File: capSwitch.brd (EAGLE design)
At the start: 45.4 x 45.7 mm, 10 parts, among them T1 2N2222, T2 2N2222

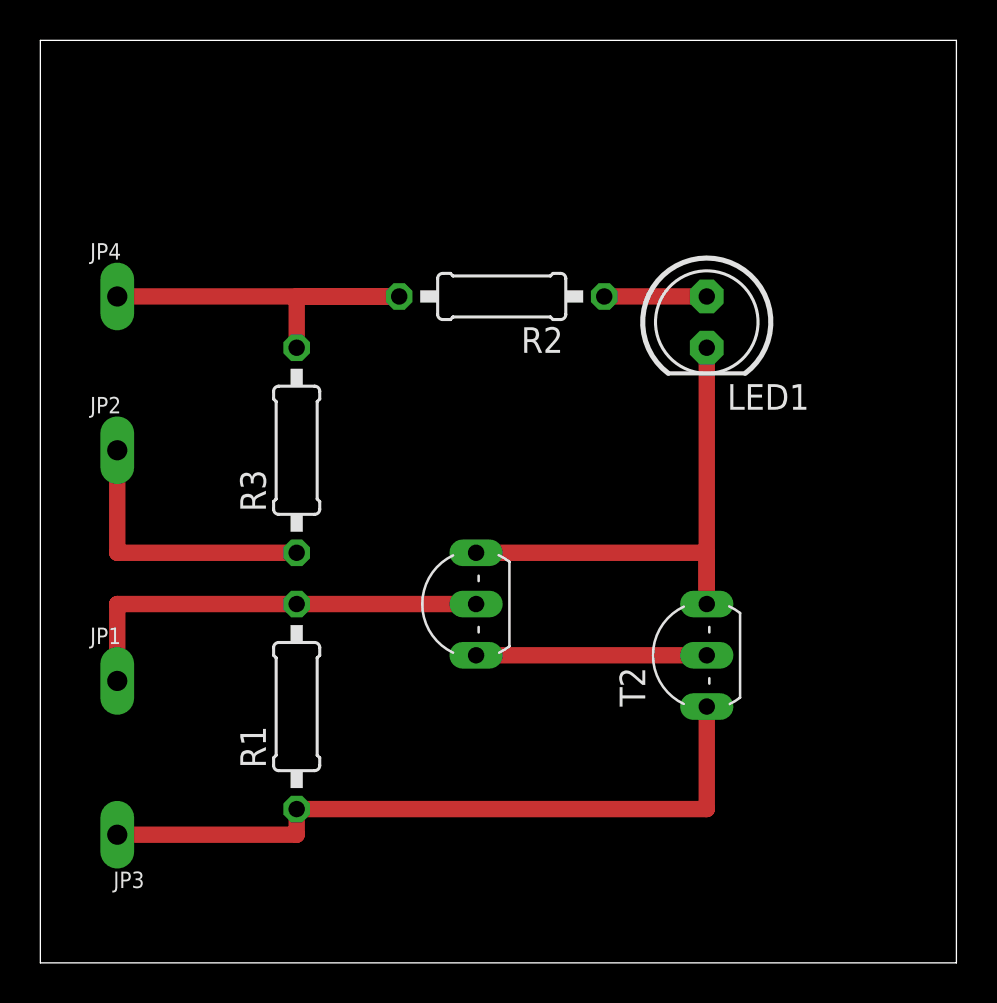
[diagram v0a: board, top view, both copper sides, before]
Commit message: refined board, ready to be etched
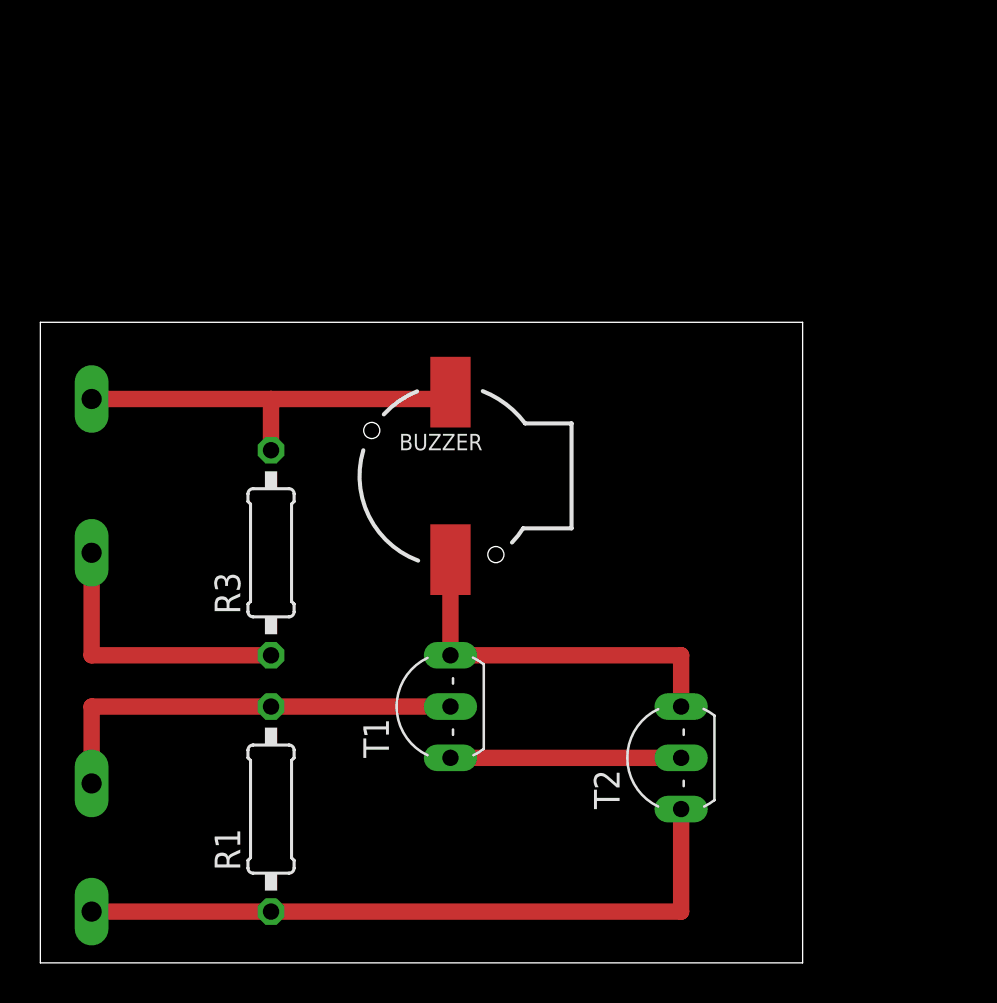
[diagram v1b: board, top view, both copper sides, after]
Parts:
- removed LED1: (no value), adafruit:LED5MM
- removed R2: 220, dp_devices:RTH025W
- added BUZZER: BUZZERSMD2-KIT, SparkFun-Electromechanical:BUZZER-CCV-KIT
- moved JP4 5.24 mm to (2.54, 27.9)
- moved T1 5.24 mm to (19.1, 12.7)
- moved JP1 5.24 mm to (2.54, 8.89)
- moved T2 5.24 mm to (30.5, 10.2)
- moved R1 5.24 mm to (11.4, 7.62)
- moved JP2 5.24 mm to (2.54, 20.3)
- moved R3 5.24 mm to (11.4, 20.3)
- moved JP3 4.02 mm to (2.54, 2.54)
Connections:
- removed net N$1: LED1.A, R2.1
- net N$2: now also BUZZER.-; no longer LED1.K
- net VCC: now also BUZZER.+; no longer R2.2
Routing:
- net N$2: track 26.7 -> 18.7 mm
- net N$1: track 5.08 -> 0.00 mm
- net GND: track 35.6 -> 34.3 mm
- net VCC: track 21.6 -> 20.7 mm
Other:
- board size 45.4 x 45.7 mm -> 37.8 x 31.7 mm
- board text added: "BUZZER"
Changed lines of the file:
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@@
 <board>
 <plain>
-<wire x1="0" y1="0" x2="45.39" y2="0" width="0" layer="20"/>
-<wire x1="45.39" y1="0" x2="45.39" y2="45.71" width="0" layer="20"/>
-<wire x1="45.39" y1="45.71" x2="0" y2="45.71" width="0" layer="20"/>
-<wire x1="0" y1="45.71" x2="0" y2="0" width="0" layer="20"/>
+<wire x1="0" y1="0" x2="37.77" y2="0" width="0" layer="20"/>
+<wire x1="37.77" y1="0" x2="37.77" y2="31.74" width="0" layer="20"/>
+<wire x1="37.77" y1="31.74" x2="0" y2="31.74" width="0" layer="20"/>
+<wire x1="0" y1="31.74" x2="0" y2="0" width="0" layer="20"/>
+<text x="17.78" y="25.4" size="0.8128" layer="21">BUZZER</text>
 </plain>
 <attributes>
@@
 </autorouter>
 <elements>
-<element name="JP1" library="microbuilder" package="1X01_OVAL" value="probe_a" x="3.81" y="13.97"/>
-<element name="JP2" library="microbuilder" package="1X01_OVAL" value="probe_b" x="3.81" y="25.4"/>
-<element name="JP3" library="microbuilder" package="1X01_OVAL" value="gnd" x="3.81" y="6.35" rot="R180"/>
-<element name="JP4" library="microbuilder" package="1X01_OVAL" value="vcc" x="3.81" y="33.02"/>
-<element name="LED1" library="adafruit" package="LED5MM" value="" x="33.02" y="31.75" smashed="yes" rot="R270">
-<attribute name="NAME" x="38.1" y="28.6766" size="1.27" layer="25" ratio="10" rot="R180"/>
-<attribute name="VALUE" x="31.2166" y="28.5496" size="1.27" layer="27" ratio="10" rot="R270"/>
-</element>
-<element name="R1" library="dp_devices" package="RTH025W" value="10M" x="12.7" y="12.7" rot="R90"/>
-<element name="R2" library="dp_devices" package="RTH025W" value="220" x="22.86" y="33.02" smashed="yes" rot="R180">
-<attribute name="NAME" x="25.908" y="31.496" size="1.27" layer="25" font="vector" ratio="10" rot="R180"/>
-<attribute name="VALUE" x="22.225" y="35.8775" size="1.27" layer="27" font="vector" ratio="10" rot="R180"/>
-</element>
-<element name="R3" library="dp_devices" package="RTH025W" value="1k" x="12.7" y="25.4" rot="R90"/>
-<element name="T1" library="adafruit" package="TO92-EBC-OVAL" value="2N2222" x="20.32" y="17.78" smashed="yes" rot="R90">
-<attribute name="VALUE" x="25.4" y="14.097" size="1.27" layer="27" ratio="10" rot="R180"/>
-</element>
-<element name="T2" library="adafruit" package="TO92-EBC-OVAL" value="2N2222" x="31.75" y="15.24" rot="R90"/>
+<element name="JP1" library="microbuilder" package="1X01_OVAL" value="probe_a" x="2.54" y="8.89" smashed="yes">
+<attribute name="VALUE" x="1.27" y="10.795" size="0.8128" layer="27" ratio="10"/>
+</element>
+<element name="JP2" library="microbuilder" package="1X01_OVAL" value="probe_b" x="2.54" y="20.32" smashed="yes">
+<attribute name="VALUE" x="5.715" y="18.415" size="0.8128" layer="27" ratio="10" rot="R180"/>
+</element>
+<element name="JP3" library="microbuilder" package="1X01_OVAL" value="gnd" x="2.54" y="2.54" smashed="yes" rot="R180">
+<attribute name="VALUE" x="3.81" y="5.08" size="0.8128" layer="27" ratio="10" rot="R180"/>
+</element>
+<element name="JP4" library="microbuilder" package="1X01_OVAL" value="vcc" x="2.54" y="27.94" smashed="yes">
+<attribute name="VALUE" x="3.81" y="26.67" size="0.8128" layer="27" ratio="10"/>
+</element>
+<element name="R1" library="dp_devices" package="RTH025W" value="10M" x="11.43" y="7.62" rot="R90"/>
+<element name="R3" library="dp_devices" package="RTH025W" value="1k" x="11.43" y="20.32" rot="R90"/>
+<element name="T1" library="adafruit" package="TO92-EBC-OVAL" value="2N2222" x="19.05" y="12.7" rot="R90"/>
+<element name="T2" library="adafruit" package="TO92-EBC-OVAL" value="2N2222" x="30.48" y="10.16" rot="R90"/>
+<element name="BUZZER" library="SparkFun-Electromechanical" package="BUZZER-CCV-KIT" value="BUZZERSMD2-KIT" x="20.32" y="24.13" rot="R90"/>
 </elements>
 <signals>
 <signal name="VCC">
 <contactref element="R3" pad="2"/>
-<contactref element="R2" pad="2"/>
 <contactref element="JP4" pad="1"/>
-<wire x1="3.81" y1="33.02" x2="17.78" y2="33.02" width="0.8128" layer="1"/>
-<wire x1="17.78" y1="33.02" x2="12.7" y2="33.02" width="0.8128" layer="1"/>
-<wire x1="12.7" y1="33.02" x2="12.7" y2="30.48" width="0.8128" layer="1"/>
-</signal>
-<signal name="N$1">
-<contactref element="LED1" pad="A"/>
-<contactref element="R2" pad="1"/>
-<wire x1="33.02" y1="33.02" x2="27.94" y2="33.02" width="0.8128" layer="1"/>
+<contactref element="BUZZER" pad="+"/>
+<wire x1="2.54" y1="27.94" x2="11.43" y2="27.94" width="0.8128" layer="1"/>
+<wire x1="11.43" y1="27.94" x2="11.43" y2="25.4" width="0.8128" layer="1"/>
+<wire x1="11.43" y1="27.94" x2="20.32" y2="27.94" width="0.8128" layer="1"/>
+<wire x1="20.32" y1="27.94" x2="20.32" y2="28.28" width="0.8128" layer="1"/>
 </signal>
 <signal name="GND">
@@
 <contactref element="T2" pad="E"/>
 <contactref element="R1" pad="1"/>
-<wire x1="12.7" y1="7.62" x2="33.02" y2="7.62" width="0.8128" layer="1"/>
-<wire x1="33.02" y1="7.62" x2="33.02" y2="12.7" width="0.8128" layer="1"/>
-<wire x1="12.7" y1="7.62" x2="12.7" y2="6.35" width="0.8128" layer="1"/>
-<wire x1="12.7" y1="6.35" x2="3.81" y2="6.35" width="0.8128" layer="1"/>
+<wire x1="11.43" y1="2.54" x2="31.75" y2="2.54" width="0.8128" layer="1"/>
+<wire x1="31.75" y1="2.54" x2="31.75" y2="7.62" width="0.8128" layer="1"/>
+<wire x1="2.54" y1="2.54" x2="11.43" y2="2.54" width="0.8128" layer="1"/>
 </signal>
 <signal name="N$3">
 <contactref element="R3" pad="1"/>
 <contactref element="JP2" pad="1"/>
-<wire x1="12.7" y1="20.32" x2="3.81" y2="20.32" width="0.8128" layer="1"/>
-<wire x1="3.81" y1="20.32" x2="3.81" y2="25.4" width="0.8128" layer="1"/>
+<wire x1="11.43" y1="15.24" x2="2.54" y2="15.24" width="0.8128" layer="1"/>
+<wire x1="2.54" y1="15.24" x2="2.54" y2="20.32" width="0.8128" layer="1"/>
 </signal>
 <signal name="N$4">
@@
 <contactref element="JP1" pad="1"/>
 <contactref element="R1" pad="2"/>
-<wire x1="12.7" y1="17.78" x2="21.59" y2="17.78" width="0.8128" layer="1"/>
-<wire x1="3.81" y1="13.97" x2="3.81" y2="17.78" width="0.8128" layer="1"/>
-<wire x1="3.81" y1="17.78" x2="12.7" y2="17.78" width="0.8128" layer="1"/>
+<wire x1="11.43" y1="12.7" x2="20.32" y2="12.7" width="0.8128" layer="1"/>
+<wire x1="2.54" y1="8.89" x2="2.54" y2="12.7" width="0.8128" layer="1"/>
+<wire x1="2.54" y1="12.7" x2="11.43" y2="12.7" width="0.8128" layer="1"/>
 </signal>
 <signal name="N$2">
 <contactref element="T2" pad="C"/>
-<contactref element="LED1" pad="K"/>
 <contactref element="T1" pad="C"/>
-<wire x1="21.59" y1="20.32" x2="33.02" y2="20.32" width="0.8128" layer="1"/>
-<wire x1="33.02" y1="20.32" x2="33.02" y2="17.78" width="0.8128" layer="1"/>
-<wire x1="33.02" y1="17.78" x2="33.02" y2="30.48" width="0.8128" layer="1"/>
+<wire x1="20.32" y1="15.24" x2="31.75" y2="15.24" width="0.8128" layer="1"/>
+<wire x1="31.75" y1="15.24" x2="31.75" y2="12.7" width="0.8128" layer="1"/>
+<contactref element="BUZZER" pad="-"/>
+<wire x1="20.32" y1="19.98" x2="20.32" y2="15.24" width="0.8128" layer="1"/>
 </signal>
 <signal name="N$6">
 <contactref element="T1" pad="E"/>
 <contactref element="T2" pad="B"/>
-<wire x1="33.02" y1="15.24" x2="21.59" y2="15.24" width="0.8128" layer="1"/>
+<wire x1="31.75" y1="10.16" x2="20.32" y2="10.16" width="0.8128" layer="1"/>
 </signal>
 </signals>
